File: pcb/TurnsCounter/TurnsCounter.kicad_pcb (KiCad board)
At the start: 2 copper layers, 69.2 x 80 mm, 42 parts, among them J1 Hall Sensors, J10 Conn_01x08_Male, J11 Conn_01x16_Male, J2 PS +9V, J3 I2C, J4 AVR-ISP-10 (SPI), J5 RGB Led, J6 RGB Led, J7 Conn_01x06_Male, J8 Keys, J9 Conn_01x08_Male, SW1 RESET, SW2 UP, SW3 CENCEL, SW4 DOWN, SW5 ENTER, U1 LM317_TO-220, U2 ATmega8A-A, U3 MAX7219

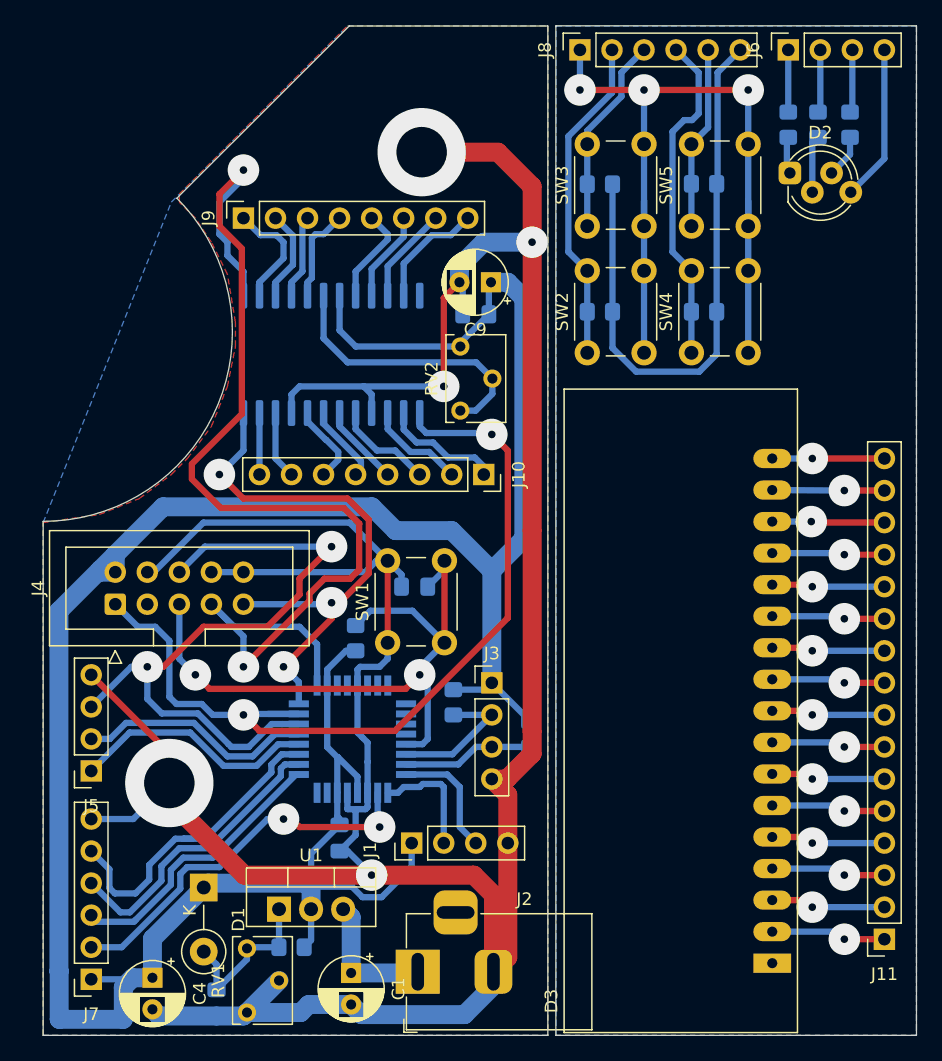
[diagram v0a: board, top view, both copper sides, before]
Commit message: pdf
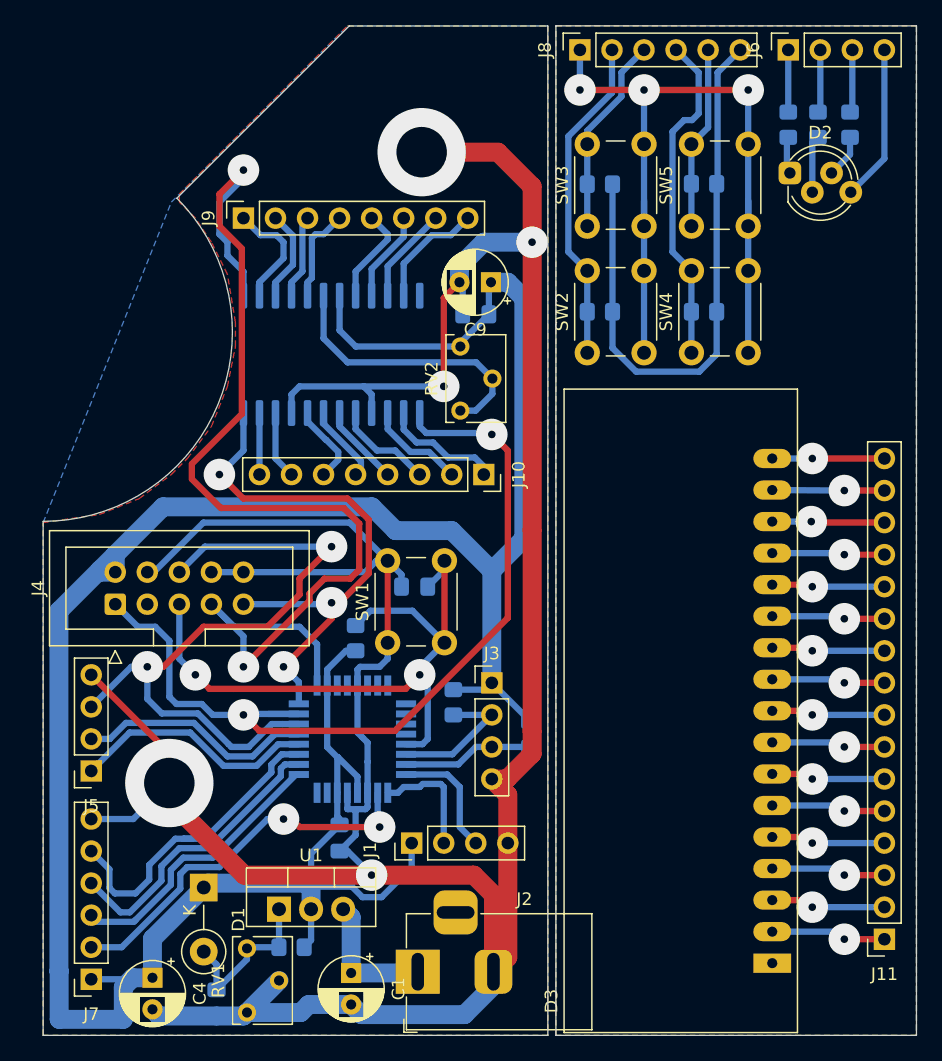
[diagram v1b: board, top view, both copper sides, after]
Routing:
- added copper zone on F.Cu, net Net-(D2-Pad4)
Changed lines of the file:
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@@
+    )
+  )
+  (zone (net 55) (net_name "Net-(D2-Pad4)") (layer "F.Cu") (hatch edge 0.508)
+    (connect_pads (clearance 0.508))
+    (min_thickness 0.254) (filled_areas_thickness no)
+    (fill yes (thermal_gap 0.508) (thermal_bridge_width 0.508))
+    (polygon
+      (pts
+        (xy 217.525 125)
+        (xy 188.95 125)
+        (xy 188.95 44.99)
+        (xy 217.525 44.99)
+      )
     )
   )
